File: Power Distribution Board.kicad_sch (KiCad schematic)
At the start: 18 parts, among them J1 XT90PW-F, J2 XT90PW-F, J3 XT90PW-F, J4 XT90PW-F, J5 SMA-J-P-H-ST-EM1, J6 XT90PW-F, J7 SMA-J-P-H-ST-EM1, U1 LM2576HVS-5

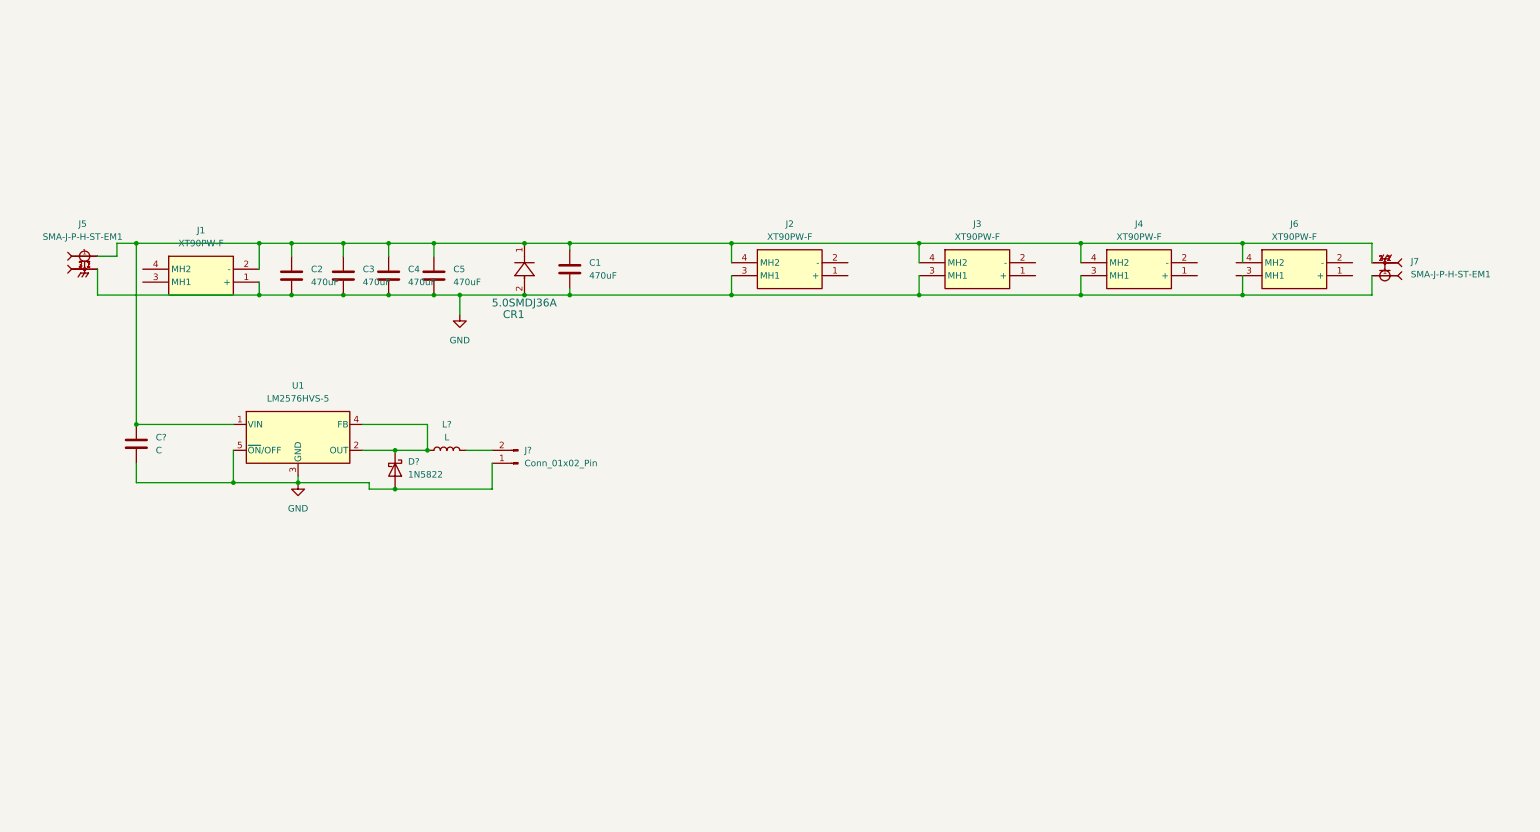
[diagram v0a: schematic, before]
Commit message: Version as of 10-16
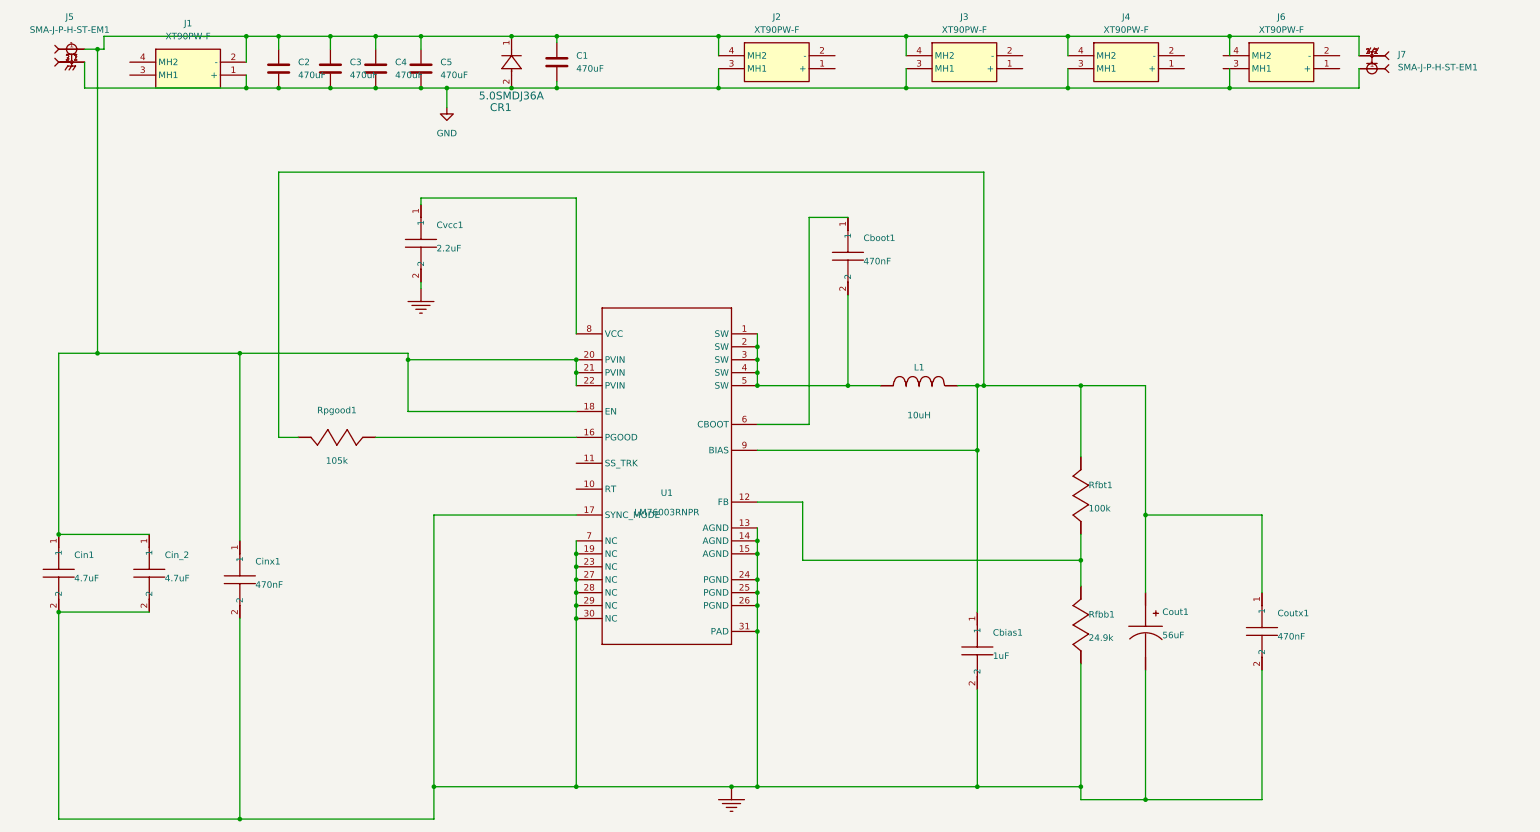
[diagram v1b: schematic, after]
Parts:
- removed C?: C, symbol Device:C
- removed D?: 1N5822, Diode_THT:D_DO-201AD_P15.24mm_Horizontal, symbol Diode:1N5822
- removed J?: Conn_01x02_Pin, symbol Connector:Conn_01x02_Pin
- removed L?: L, symbol Device:L
- removed U1: LM2576HVS-5, Package_TO_SOT_SMD:TO-263-5_TabPin3, symbol Regulator_Switching:LM2576HVS-5
- added Cbias1: C0603C105K8PACTU, symbol TI WEBENCH:root_1_Cbias_TI WEBENCH
- added Cboot1: GRM155R60J474KE19D, symbol TI WEBENCH:root_1_Cboot_TI WEBENCH
- added Cin1: GCM32DC72A475KE02L, symbol TI WEBENCH:root_1_Cin_TI WEBENCH
- added Cin_2: GCM32DC72A475KE02L, symbol TI WEBENCH:root_1_Cin_2_TI WEBENCH
- added Cinx1: MSASH21GSB5474KTCA01, symbol TI WEBENCH:root_1_Cinx_TI WEBENCH
- added Cout1: APXE100ARA560ME61G, symbol TI WEBENCH:root_1_Cout_TI WEBENCH
- added Coutx1: C1608X6S1H474K080AB, symbol TI WEBENCH:root_1_Coutx_TI WEBENCH
- added Cvcc1: GRM21BR71A225KA01L, symbol TI WEBENCH:root_1_Cvcc_TI WEBENCH
- added L1: 10uH, Inductor_SMD:L_APV_APH1030, symbol TI WEBENCH:root_0_L1_TI WEBENCH
- added Rfbb1: CRCW040224K9FKED, symbol TI WEBENCH:root_1_Rfbb_TI WEBENCH
- added Rfbt1: CRCW0402100KFKED, symbol TI WEBENCH:root_1_Rfbt_TI WEBENCH
- added Rpgood1: RC0201FR-07105KL, symbol TI WEBENCH:root_2_Rpgood_TI WEBENCH
- added U1: LM76003RNPR, LM76003RNPT:RNP0030B, symbol TI WEBENCH:root_0_U1_TI WEBENCH
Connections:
- net at C1.1, C2.1, C3.1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: now also Cin1.1, Cin_2.1, Cinx1.1, U1.18 (EN), U1.20 (PVIN), U1.21 (PVIN), U1.22 (PVIN)
- new net: Cboot1.1, U1.6 (CBOOT)
- new net: Cboot1.2, L1.1, U1.1 (SW), U1.2 (SW), U1.3 (SW), U1.4 (SW), U1.5 (SW)
- new net: Cbias1.1, Cout1.1 (+), Coutx1.1, L1.2, Rfbt1.1, Rpgood1.1, U1.9 (BIAS)
- new net: Rfbb1.1, Rfbt1.2, U1.12 (FB)
- new net: Rpgood1.2, U1.16 (PGOOD)
- new net: Cvcc1.1, U1.8 (VCC)
- new net 0: Cbias1.2, Cin1.2, Cin_2.2, Cinx1.2, Cout1.2 (-), Coutx1.2, Cvcc1.2, Rfbb1.2, U1.13 (AGND), U1.14 (AGND), U1.15 (AGND), U1.17 (SYNC_MODE), U1.19 (NC), U1.23 (NC), U1.24 (PGND), U1.25 (PGND), U1.26 (PGND), U1.27 (NC), U1.28 (NC), U1.29 (NC), U1.30 (NC), U1.31 (PAD), U1.7 (NC)
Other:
- moved on the sheet: C1, C2, C3, C4, C5, CR1, J1, J2, J3, J4, J5, J6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
